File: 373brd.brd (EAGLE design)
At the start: 160 x 100 mm, 40 parts, among them U3 XC6210

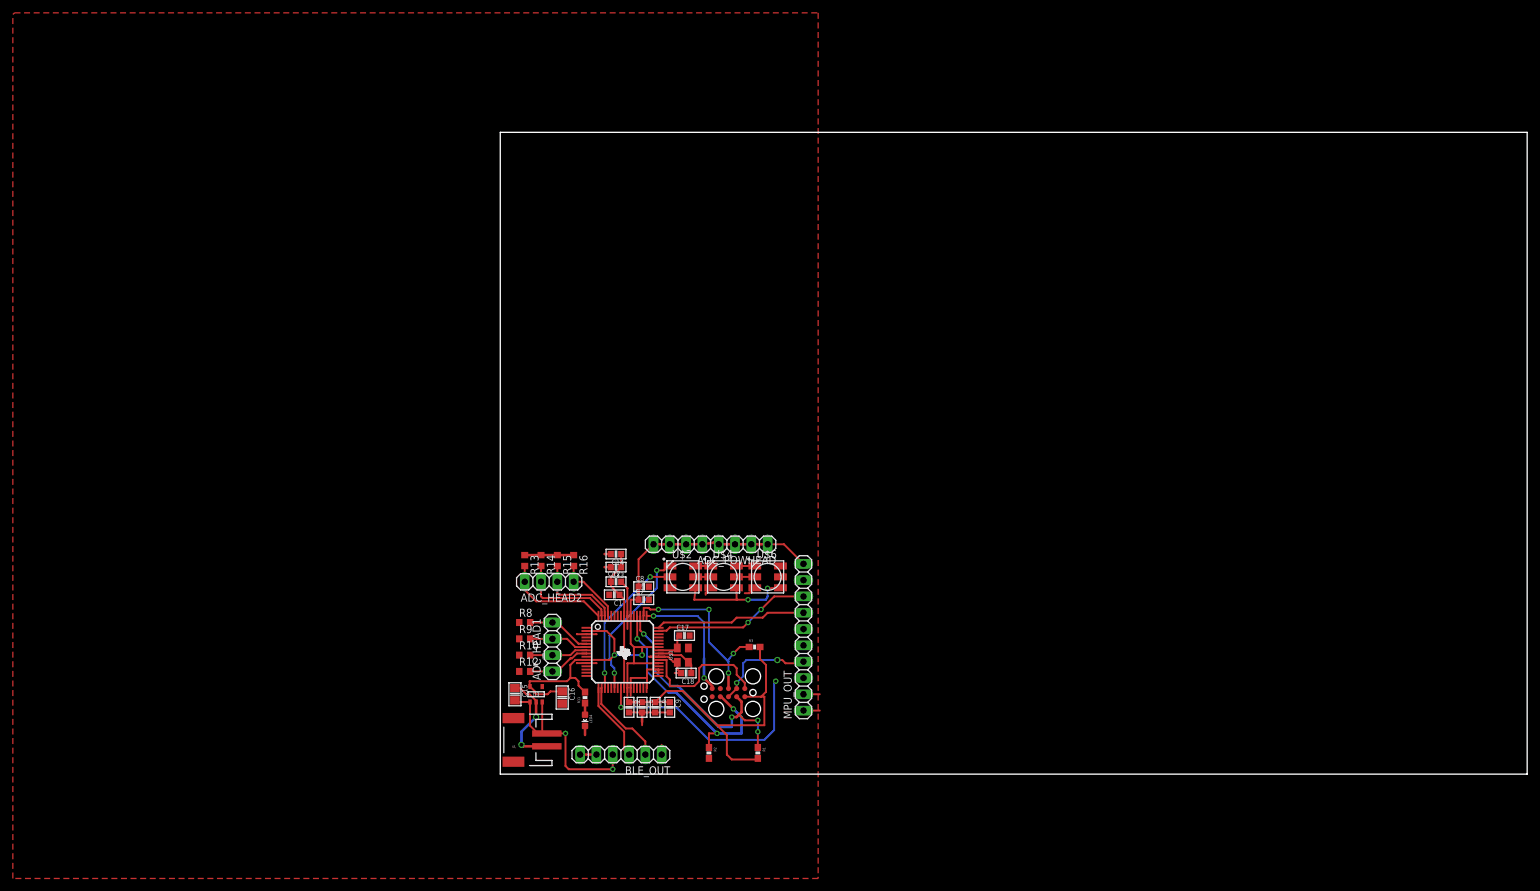
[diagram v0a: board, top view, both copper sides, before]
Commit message: done for real
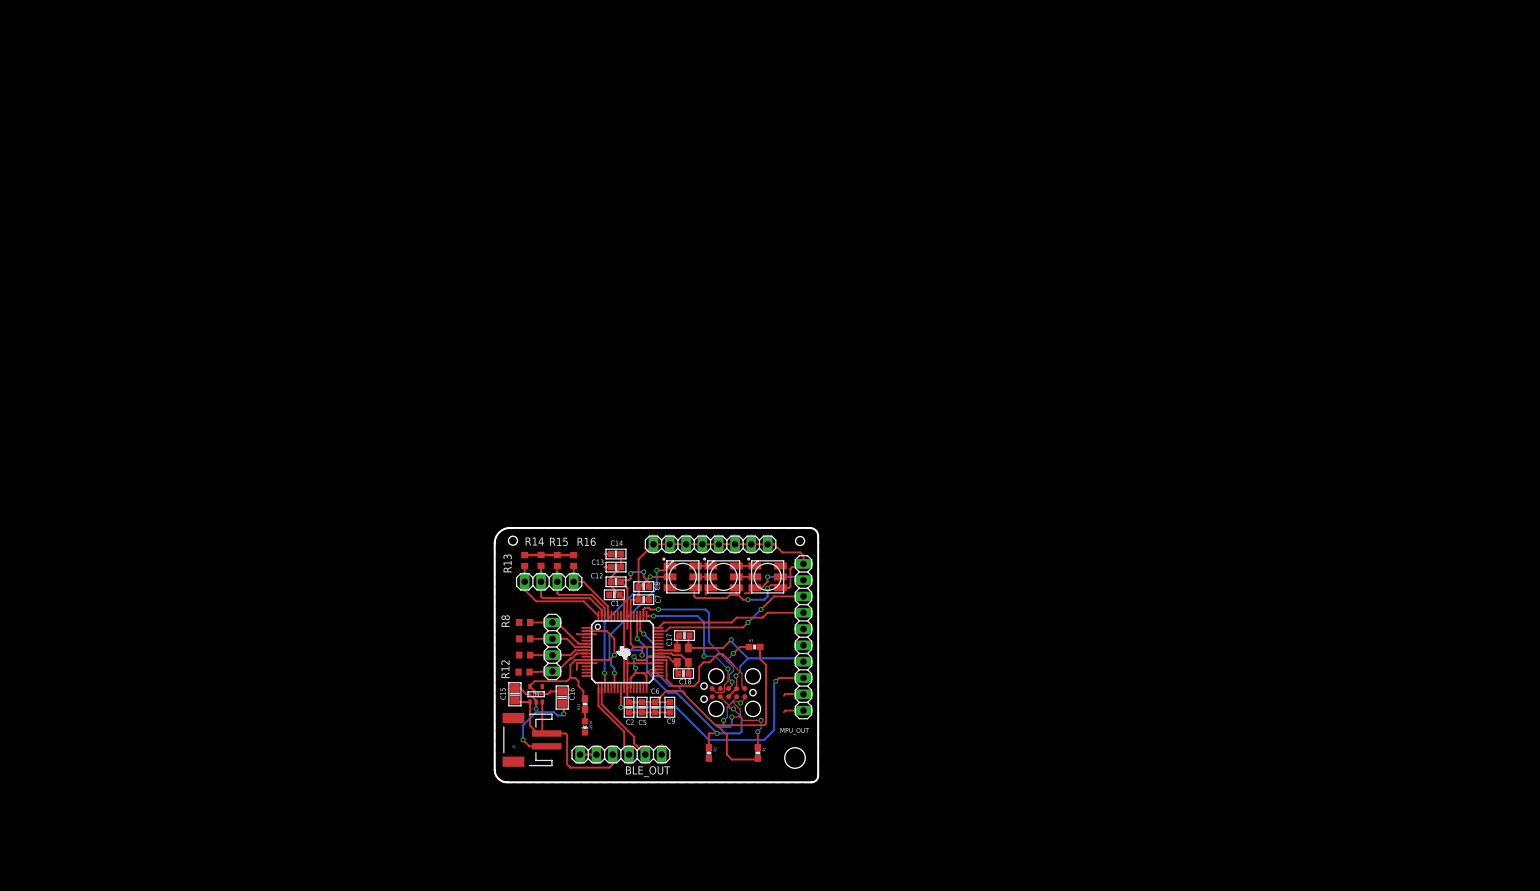
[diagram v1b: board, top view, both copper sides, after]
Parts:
- moved LED4 1.02 mm to (13.2, 7.37)
- moved R11 1.02 mm to (13.2, 10.9)
- moved C18 0.41 mm to (28.5, 15.7)
- moved R12 0.14 mm to (3.71, 15.9)
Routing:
- net GND: track 98.6 -> 138.7 mm, vias 4 -> 10
- net +3V3: track 171.4 -> 184.7 mm, vias 4 -> 6
- net PC3/TDO/SWO: track 20.2 -> 25.2 mm, vias 2 -> 3
- net MPU_INT: track 38.4 -> 42.9 mm
- net RESET: track 22.4 -> 24.0 mm
- net PC1/TMS/SWDIO: track 38.7 -> 40.1 mm
- net BATT_IN: track 32.0 -> 31.1 mm, vias 2 -> 0
- net BLE_UART_TX: track 13.9 -> 13.2 mm
- net PC2/TDI: track 29.4 -> 30.1 mm, vias 4 -> 3
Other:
- board size 160 x 100 mm -> 50.4 x 39.6 mm
- board text added: "GloveBoard, rev0 Designed by James Connolly Laid out by James Connolly"
